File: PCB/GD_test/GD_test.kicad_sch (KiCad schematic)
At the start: 47 parts, among them J4 RF_IN, J5 Conn_01x01_Pin, J6 Conn_01x01_Pin, Q1 EPC2051, Q2 EPC2051, Q3 GS61004B-MR, Q5 EPC2014C, U1 LMG1020YFF, U1 TLV3501, U11 LMG1020YFF, U3 NC7WZ04, U5 NC7WZ04, U6 NC7WZ04, U7 NC7WZ04, U9 LMG1020YFF

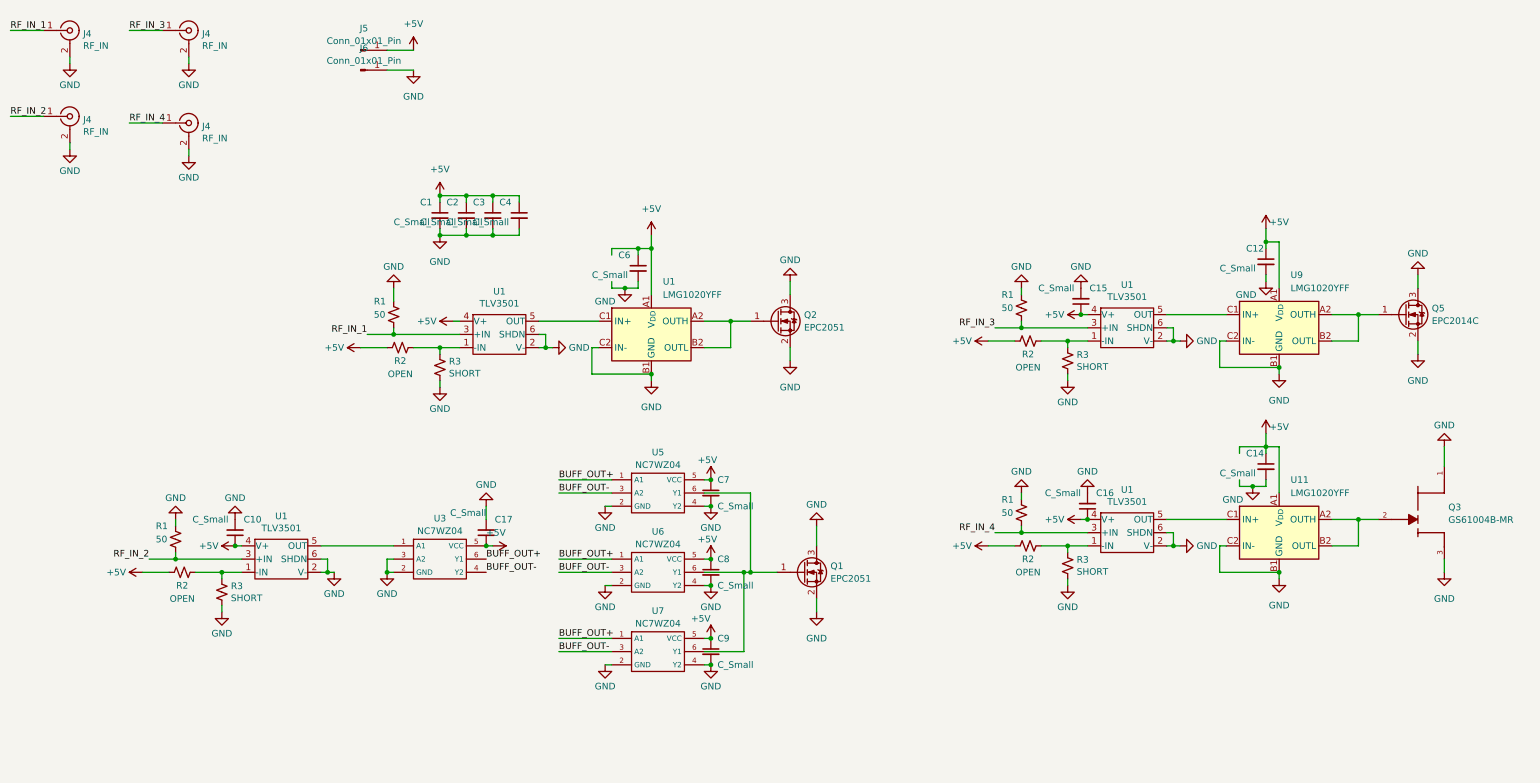
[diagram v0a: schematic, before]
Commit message: gate driver testboard rev 3 stuff
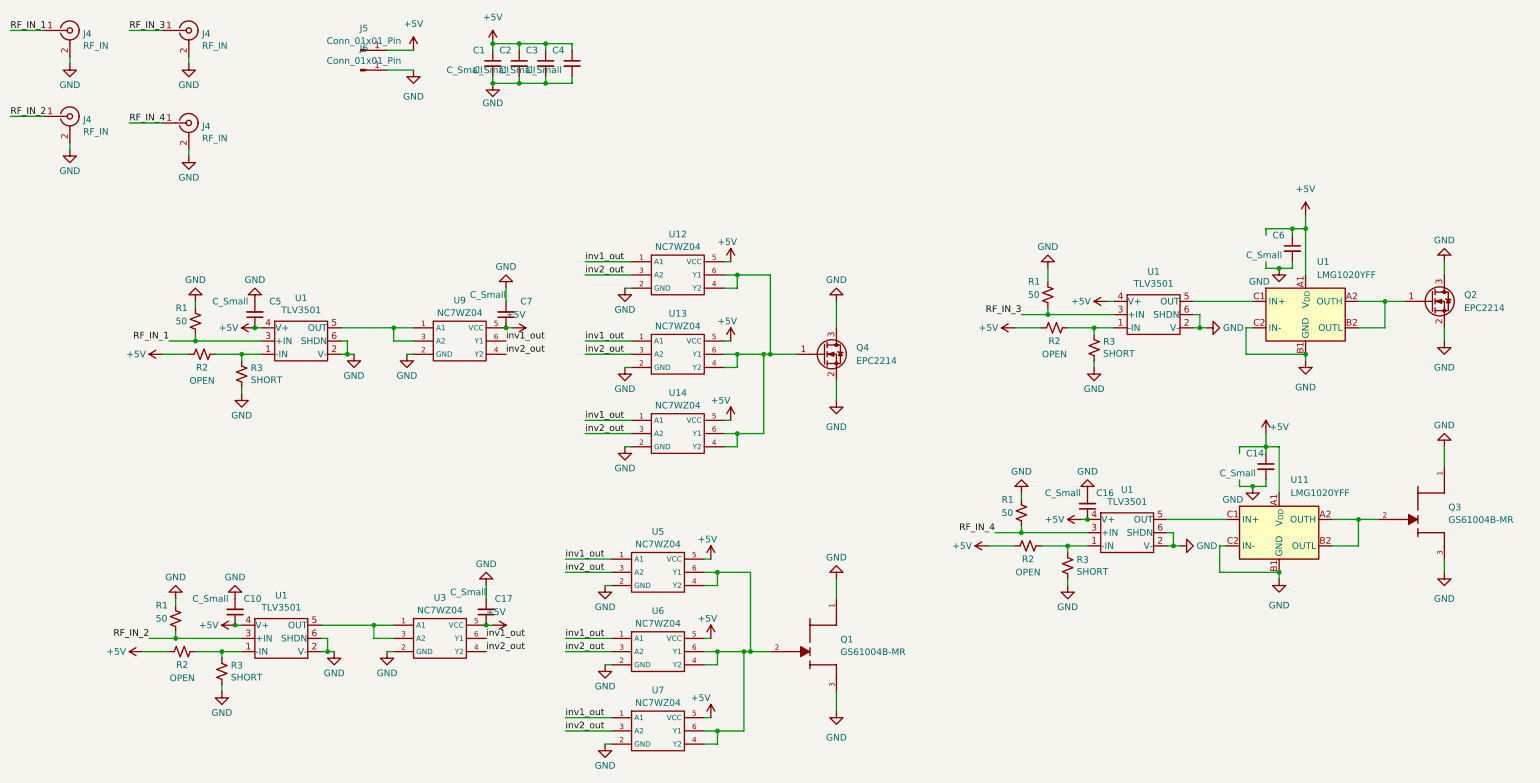
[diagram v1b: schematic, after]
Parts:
- removed C12, C15: C_Small, Capacitor_SMD:C_0603_1608Metric_Pad1.08x0.95mm_HandSolder, symbol Device:C_Small
- removed C8, C9: C_Small, Capacitor_SMD:C_0402_1005Metric_Pad0.74x0.62mm_HandSolder, symbol Device:C_Small
- removed Q1: EPC2051, EPCGaN:BGA-6_3x2_6.0x6.0mm, symbol Device:Q_NMOS_GSD
- removed Q5: EPC2014C, EPCGaN:EPC2014C, symbol Device:Q_NMOS_GSD
- removed U9: LMG1020YFF, GateDriver:BGA6N40P3X2_125X85X62N, symbol Driver_FET:LMG1020YFF
- added C5: C_Small, Capacitor_SMD:C_0603_1608Metric, symbol Device:C_Small
- added Q1: GS61004B-MR, GS61004B-MR:TRANS_GS61004B-MR, symbol GS61004B-MR:GS61004B-MR
- added Q4: EPC2214, EPCGaN:BGA-6_3x2_6.0x6.0mm, symbol Device:Q_NMOS_GSD
- added U12, U13, U14, U9: NC7WZ04, pcbparts:SOIC-6, symbol parts:NC7WZ04
- C1, C10, C14, C16, C2, C3, C4: footprint Capacitor_SMD:C_0603_1608Metric_Pad1.08x0.95mm_HandSolder -> Capacitor_SMD:C_0603_1608Metric
- C17, C6, C7: footprint Capacitor_SMD:C_0402_1005Metric_Pad0.74x0.62mm_HandSolder -> Capacitor_SMD:C_0402_1005Metric
- Q2: value EPC2051 -> EPC2214
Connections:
- net +5V: now also C5.1, U12.5 (VCC), U13.5 (VCC), U14.5 (VCC), U9.5 (VCC)
- net GND: now also C5.2, Q1.1, Q1.3, Q4.2 (S), Q4.3 (D), Q4.4 (D), Q4.5 (D), Q4.6 (D), U12.2 (GND), U13.2 (GND), U14.2 (GND), U9.2 (GND); no longer U3.3 (A2), U5.4 (Y2), U6.4 (Y2), U7.4 (Y2)
- net RF_IN_1: now also R1.2, U1.3 (+IN); no longer R1.2, U1.3 (+IN)
- net RF_IN_3: now also R1.2, U1.3 (+IN); no longer R1.2, U1.3 (+IN)
- net at U5.6 (Y1), U6.6 (Y1), U7.6 (Y1): now also U5.4 (Y2), U6.4 (Y2), U7.4 (Y2), Q1.2
- net at U1.5 (OUT): now also U9.1 (A1), U9.3 (A2)
- net at U1.5 (OUT), U3.1 (A1): now also U3.3 (A2)
- net BUFF_OUT+ renamed inv1_out
- net inv1_out: now also U12.1 (A1), U13.1 (A1), U14.1 (A1), U9.6 (Y1)
- net BUFF_OUT- renamed inv2_out
- net inv2_out: now also U12.3 (A2), U13.3 (A2), U14.3 (A2), U9.4 (Y2)
- new net: Q4.1 (G), U12.4 (Y2), U12.6 (Y1), U13.4 (Y2), U13.6 (Y1), U14.4 (Y2), U14.6 (Y1)
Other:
- moved on the sheet: C1, C10, C17, C2, C3, C4, C6, Q2, R1, R2, R3, U1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
